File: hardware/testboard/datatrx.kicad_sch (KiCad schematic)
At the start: 11 parts, among them U16 SN74ALVC164245, U17 SN74ALVC164245

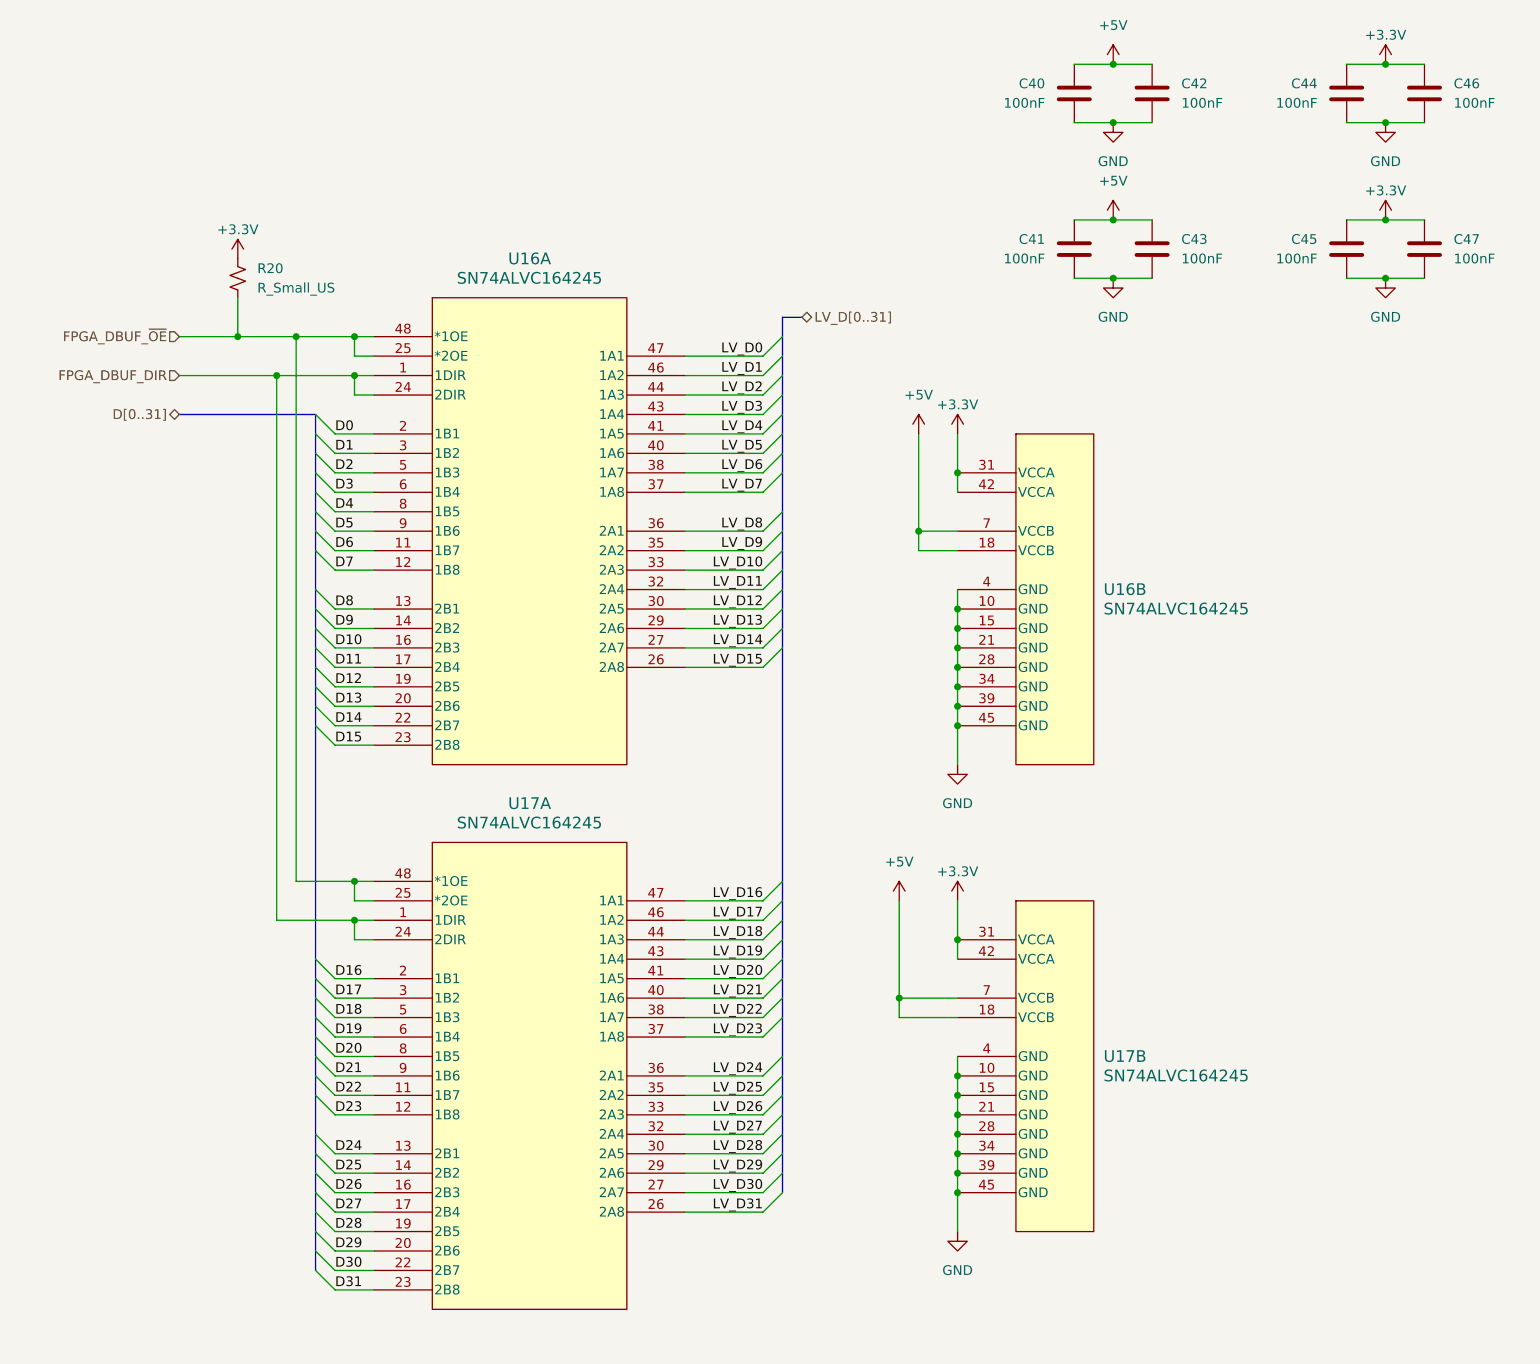
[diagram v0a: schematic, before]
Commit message: simpleboard nearly complete
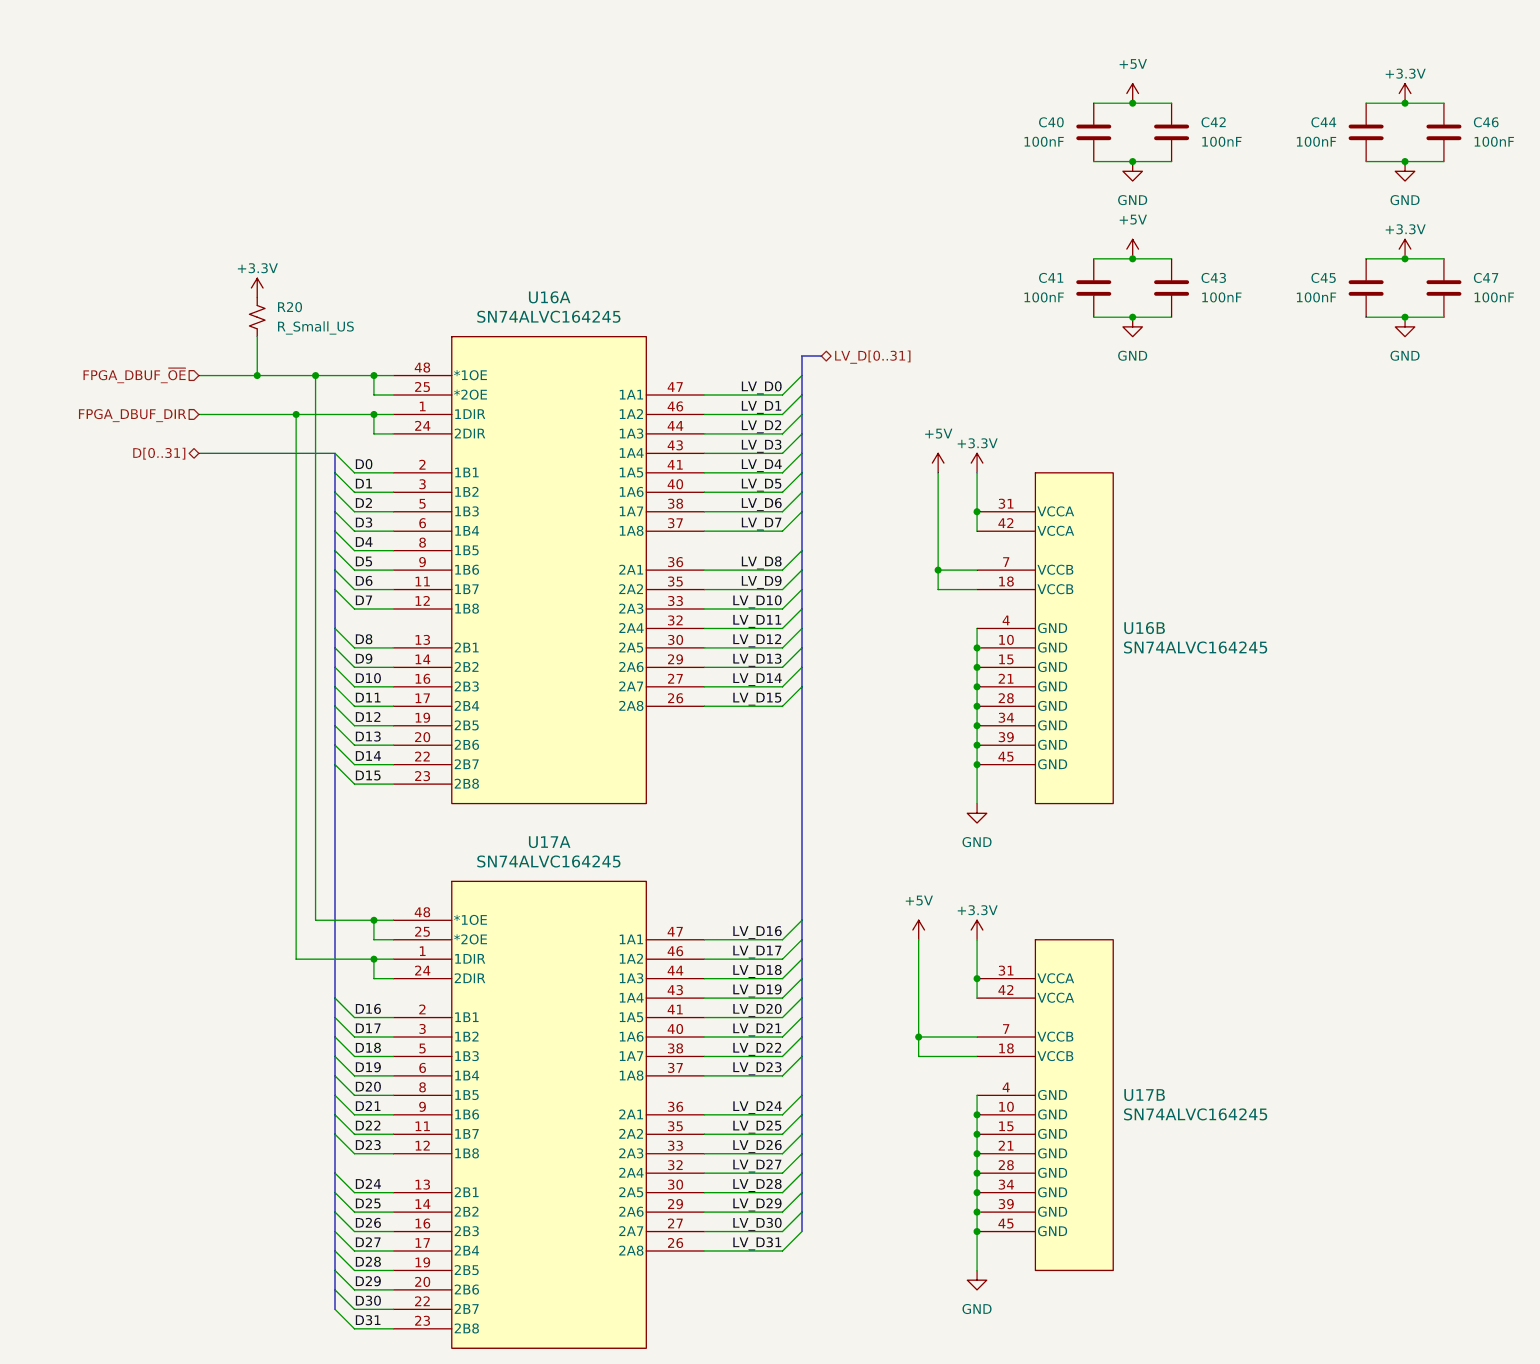
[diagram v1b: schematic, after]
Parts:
- C40, C41, C42, C43, C44, C45, C46, C47: footprint (none) -> Capacitor_SMD:C_0603_1608Metric
- R20: footprint (none) -> Resistor_SMD:R_0603_1608Metric
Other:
- moved on the sheet: C40, C41, C42, C43, C44, C45, C46, C47, R20, U16A, U16B, U17A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
